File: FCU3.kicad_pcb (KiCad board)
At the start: 4 copper layers, 36.7 x 36.7 mm, 54 parts, among them J1 SM06B-SRSS-TB_LF__SN_, J2 SM06B-SRSS-TB_LF__SN_, J4 SM08B-SRSS-TB_LF__SN_, J6 UJ20-C-H-G-SMT-1-P16-TR, Q2 SS8050, U1 MPU-6500, U3 MCP1700x-330xxTT, U5 STM32F405RGTx, Y1 LFXTAL055207Bulk

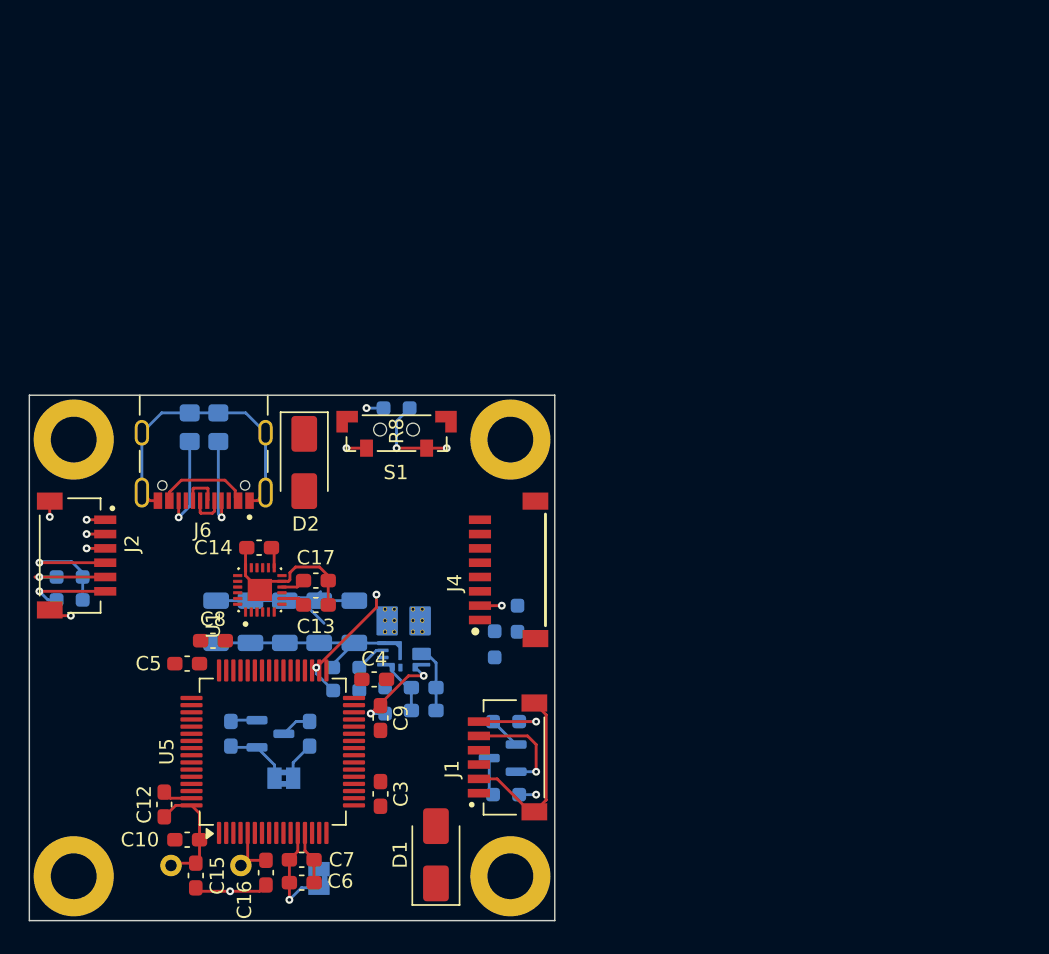
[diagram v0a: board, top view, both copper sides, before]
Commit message: Floor Plan Complete
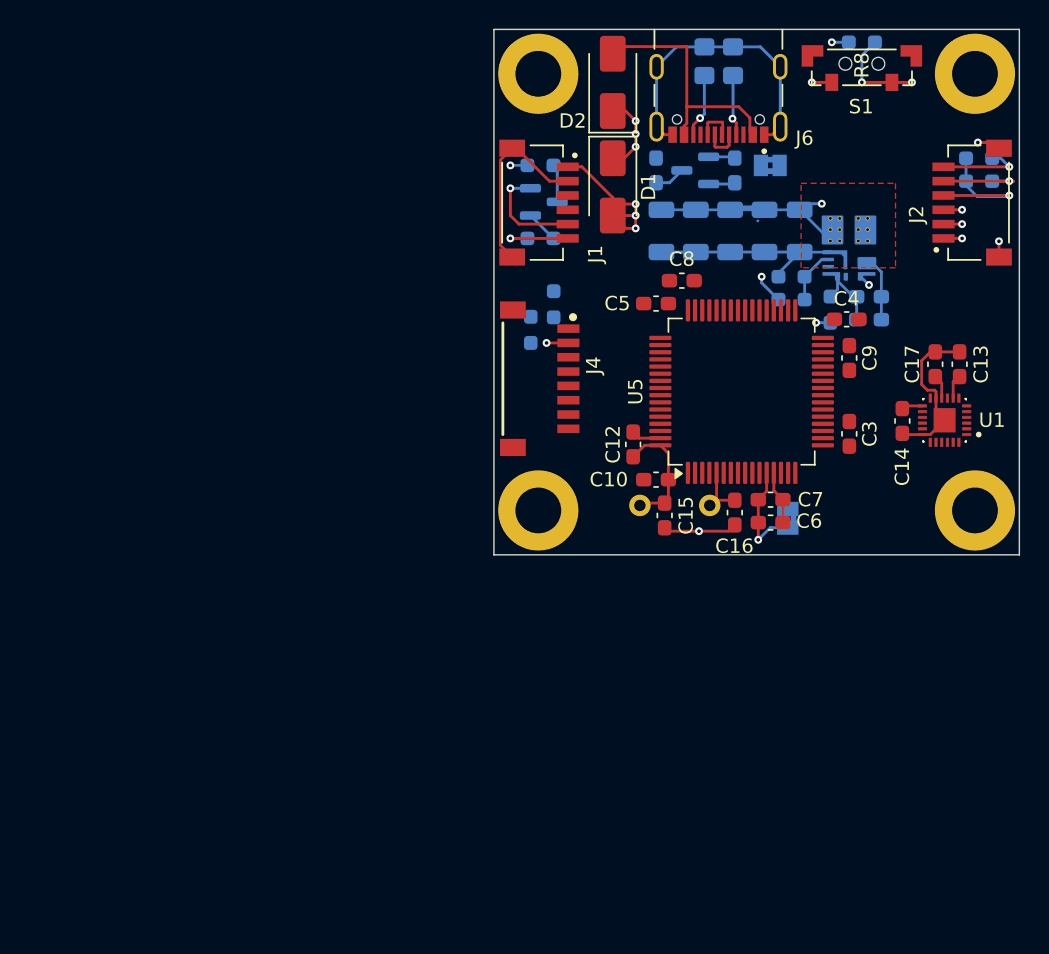
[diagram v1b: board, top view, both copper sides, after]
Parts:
- moved R10 70.6 mm to (163.2, 80.3), turned to 180 degrees
- moved R7 69.3 mm to (163.2, 82.0), turned to 180 degrees
- moved J2 63.5 mm to (160.8, 83.5), turned to 90 degrees
- moved JP4 54.6 mm to (148.7, 80.8)
- moved C2 52.8 mm to (146.2, 81.2), turned to 90 degrees
- moved U3 49.3 mm to (143.4, 81.2), turned to 180 degrees
- moved U1 49.3 mm to (160.8, 98.7), turned to 180 degrees
- moved D1 48.3 mm to (137.7, 82.3), turned to -90 degrees
- moved C13 48.0 mm to (161.9, 94.7), turned to 90 degrees
- moved C1 46.2 mm to (140.7, 81.2), turned to 90 degrees
- moved C17 45.8 mm to (160.2, 94.7), turned to 90 degrees
- moved C14 45.8 mm to (157.9, 98.7), turned to -90 degrees
- moved R15 44.1 mm to (144.1, 73.6)
- moved R9 44.1 mm to (146.1, 73.6)
- moved J6 44.1 mm to (145.0, 71.4)
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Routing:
- net /Project Architecture/V_USB: track 6.64 -> 17.6 mm
- net +9V: track 22.8 -> 29.6 mm, vias 2 -> 5
- net Net-(D1-K): track 2.16 -> 7.78 mm, vias 0 -> 3
- net Net-(PS1-MODE): track 6.64 -> 1.85 mm
- net PGND: track 56.0 -> 53.3 mm
- net DGND: track 36.4 -> 33.8 mm
- net /Project Architecture/USB_CC1: track 6.68 -> 4.30 mm
- net /Project Architecture/USB_CC2: track 6.79 -> 4.45 mm
- added copper zone on F.Cu, net +9V
- added copper zone on In1.Cu, net DGND
- added copper zone on In2.Cu, net PGND
